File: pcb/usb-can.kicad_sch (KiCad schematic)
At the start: 54 parts, among them J1 Micro_SD_Card_Det1, J2 Conn_ARM_SWD_TagConnect_TC203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, J3 USB_C_Receptacle_USB2.0_16P, J4 Conn_01x04_MountingPin, J5 Conn_01x04_MountingPin, U1 STM32G473CBTx, U2 TJA1042T-3, U3 SRV05-4, U4 AMS1117-3.3, U5 TPS5430DDA, Y1 16MHz

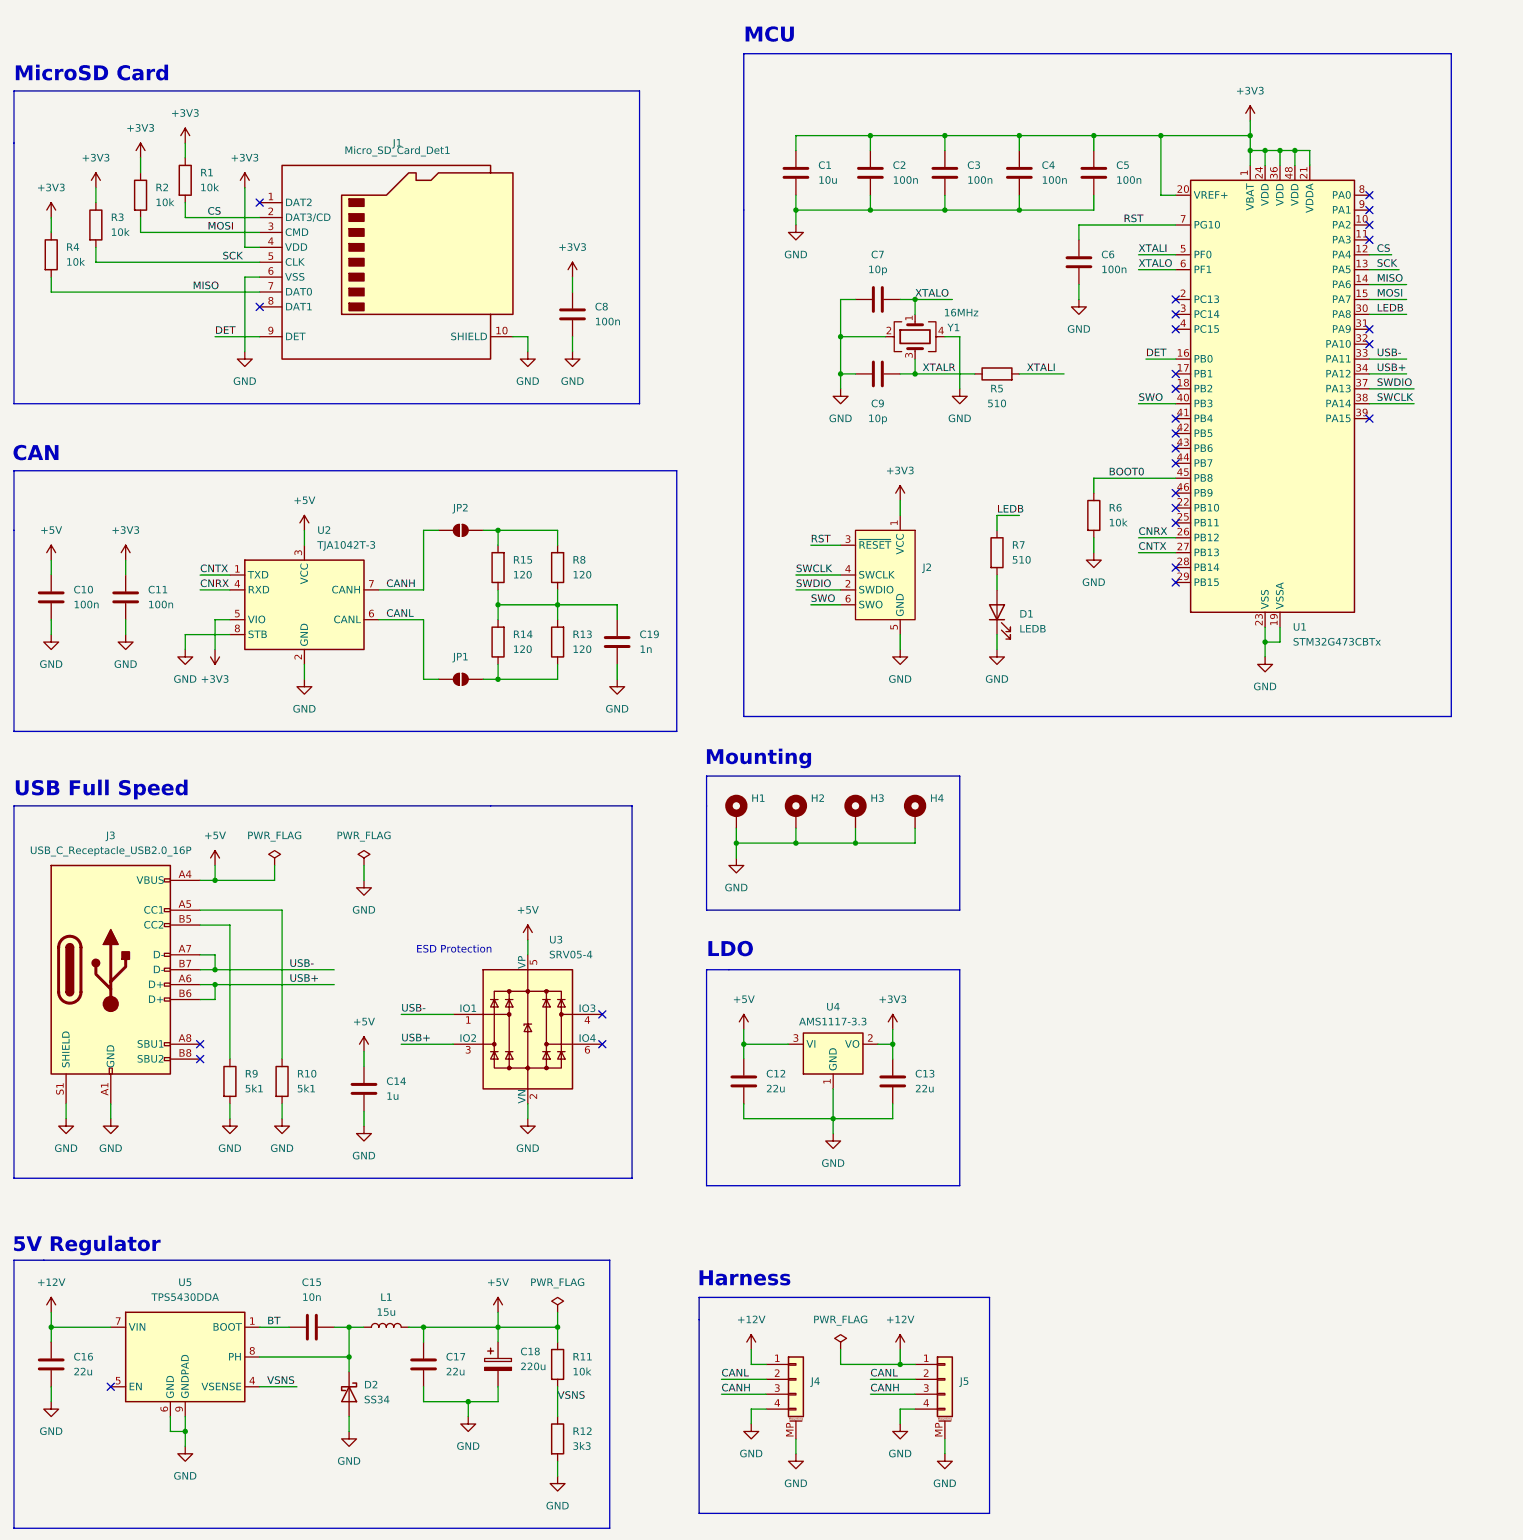
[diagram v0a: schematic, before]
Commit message: Minimize schematic
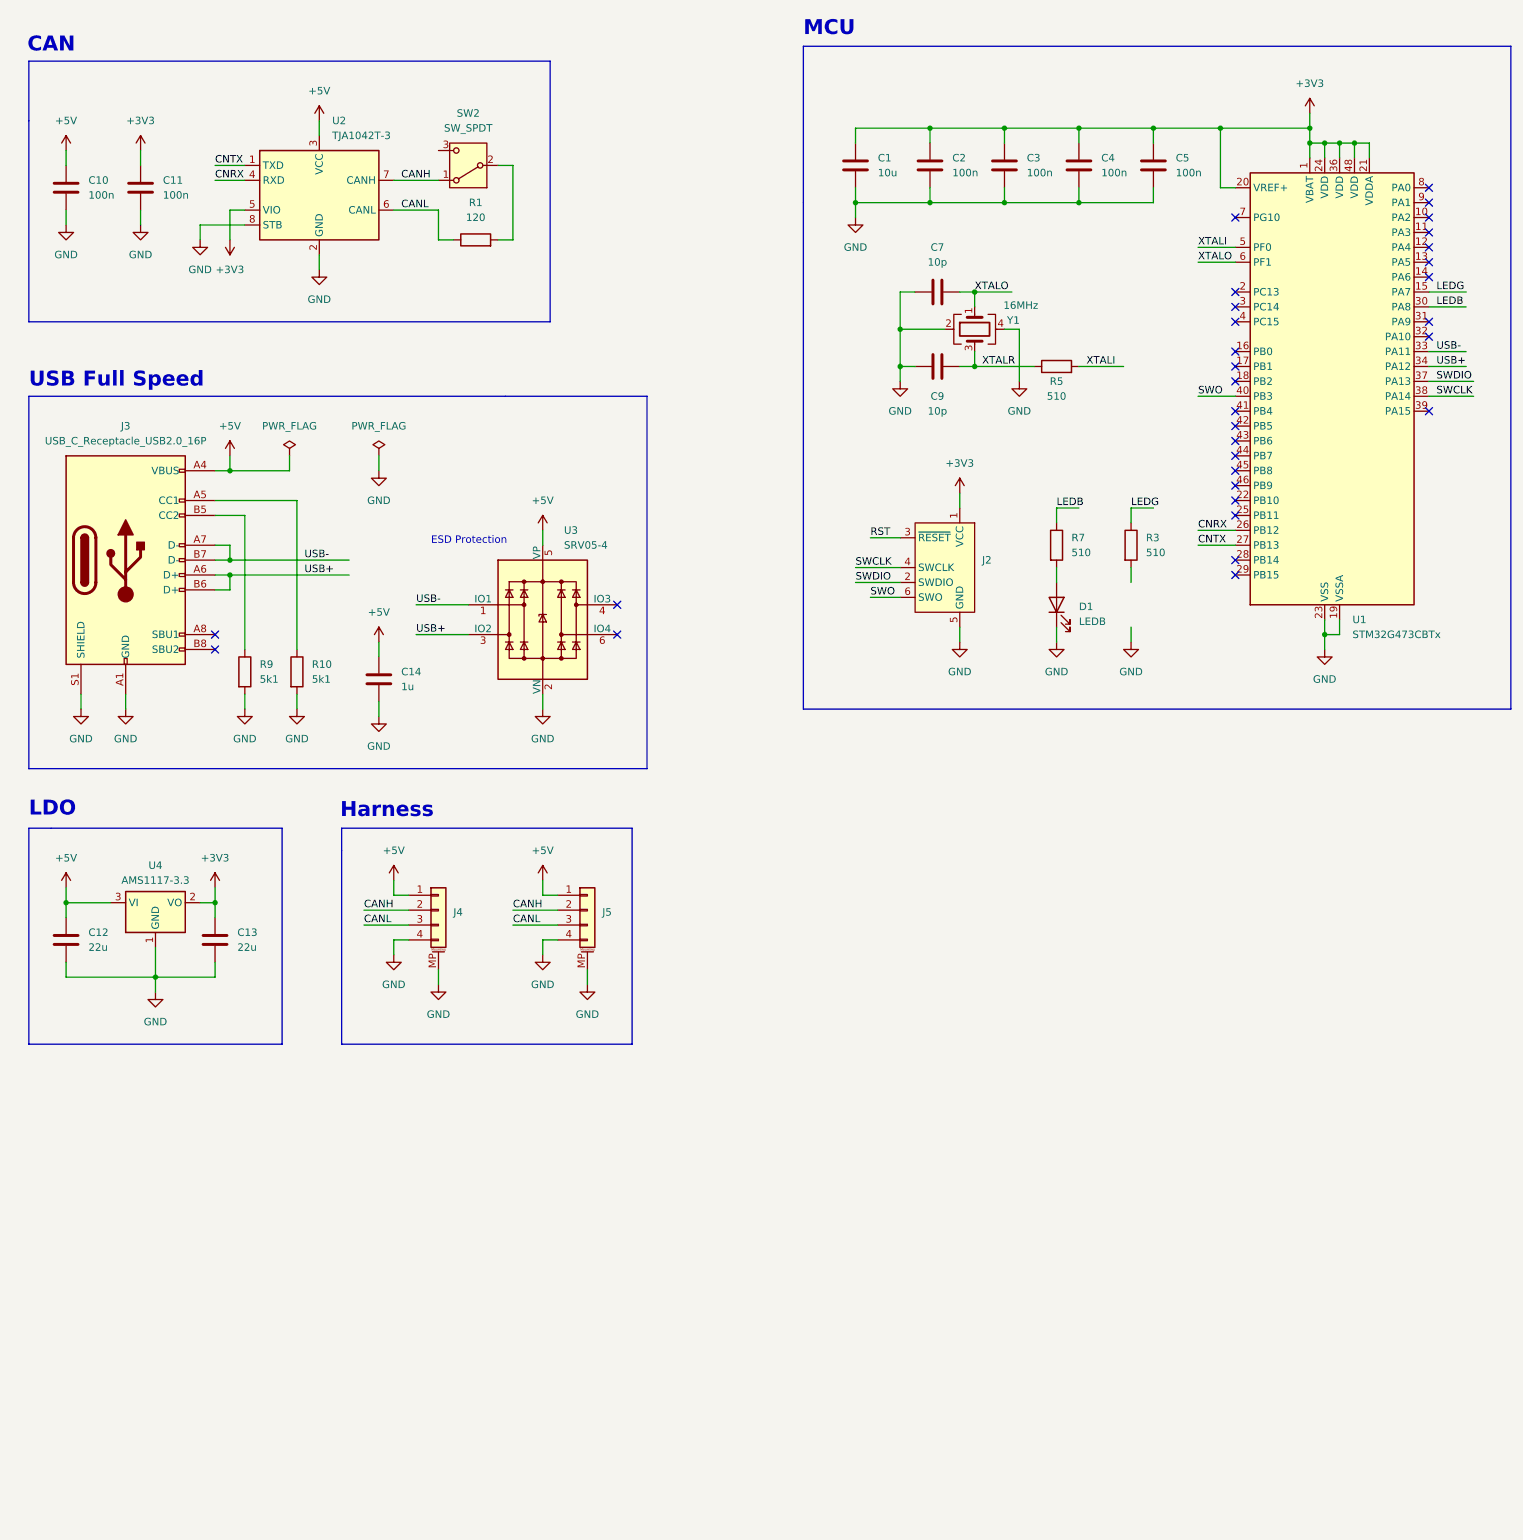
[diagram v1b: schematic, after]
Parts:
- removed C15: 10n, Capacitor_SMD:C_0402_1005Metric, symbol Device:C
- removed C16, C17: 22u, Capacitor_SMD:C_1206_3216Metric, symbol Device:C
- removed C18: 220u, Capacitor_SMD:CP_Elec_6.3x5.4, symbol Device:C_Polarized
- removed C19: 1n, Capacitor_SMD:C_0603_1608Metric, symbol Device:C
- removed C6, C8: 100n, Capacitor_SMD:C_0402_1005Metric, symbol Device:C
- removed D2: SS34, Diode_SMD:D_SMA, symbol Device:D_Schottky
- removed H1, H2, H3, H4: MountingHole_Pad, MountingHole:MountingHole_3.2mm_M3_ISO7380_Pad, symbol Mechanical:MountingHole_Pad
- removed J1: Micro_SD_Card_Det1, User_Footprints:SD-CARD, symbol Connector:Micro_SD_Card_Det1
- removed JP1, JP2: SolderJumper_2_Open, Jumper:SolderJumper-2_P1.3mm_Open_RoundedPad1.0x1.5mm, symbol Jumper:SolderJumper_2_Open
- removed L1: 15u, Inductor_SMD:L_Sunlord_MWSA0503S, symbol Device:L
- removed R11, R2, R4, R6: 10k, Resistor_SMD:R_0402_1005Metric, symbol Device:R
- removed R12: 3k3, Resistor_SMD:R_0402_1005Metric, symbol Device:R
- removed R13, R14, R15, R8: 120, Resistor_SMD:R_0603_1608Metric, symbol Device:R
- removed U5: TPS5430DDA, Package_SO:TI_SO-PowerPAD-8_ThermalVias, symbol Regulator_Switching:TPS5430DDA
- added SW2: SW_SPDT, symbol Switch:SW_SPDT
- R1: value 10k -> 120; footprint Resistor_SMD:R_0402_1005Metric -> Resistor_SMD:R_1206_3216Metric; LCSC C25744 -> C17909
- R3: value 10k -> 510; LCSC C25744 -> C25123
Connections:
- net +12V is gone; now on net +5V: J4.1 (Pin_1), J5.1 (Pin_1)
- net +3V3: no longer R1.1, R3.1
- net CANH: now also J4.2 (Pin_2), J5.2 (Pin_2), SW2.1 (A); no longer J4.3 (Pin_3), J5.3 (Pin_3)
- net CANL: now also J4.3 (Pin_3), J5.3 (Pin_3), R1.1; no longer J4.2 (Pin_2), J5.2 (Pin_2)
- net RST: no longer U1.7 (PG10)
- net BOOT0: no longer names the net of U1.45 (PB8)
- net CS: no longer names the net of R1.2
- net CS: now also SW2.2 (B); no longer U1.12 (PA4)
- net DET: no longer names the net of U1.16 (PB0)
- net MISO: no longer names the net of U1.14 (PA6)
- net MOSI renamed LEDG
- net LEDG: now also R3.1
- net SCK: no longer names the net of U1.13 (PA5)
- net SCK: no longer R3.2
- no-connect marks 28 -> 31
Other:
- note removed: "5V Regulator"
- note removed: "MicroSD Card"
- note removed: "Mounting"
- moved on the sheet: C1, C10, C11, C12, C13, C14, C2, C3, C4, C5, C7, C9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
